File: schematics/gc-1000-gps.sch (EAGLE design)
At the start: 17 parts, among them T1 2N3904

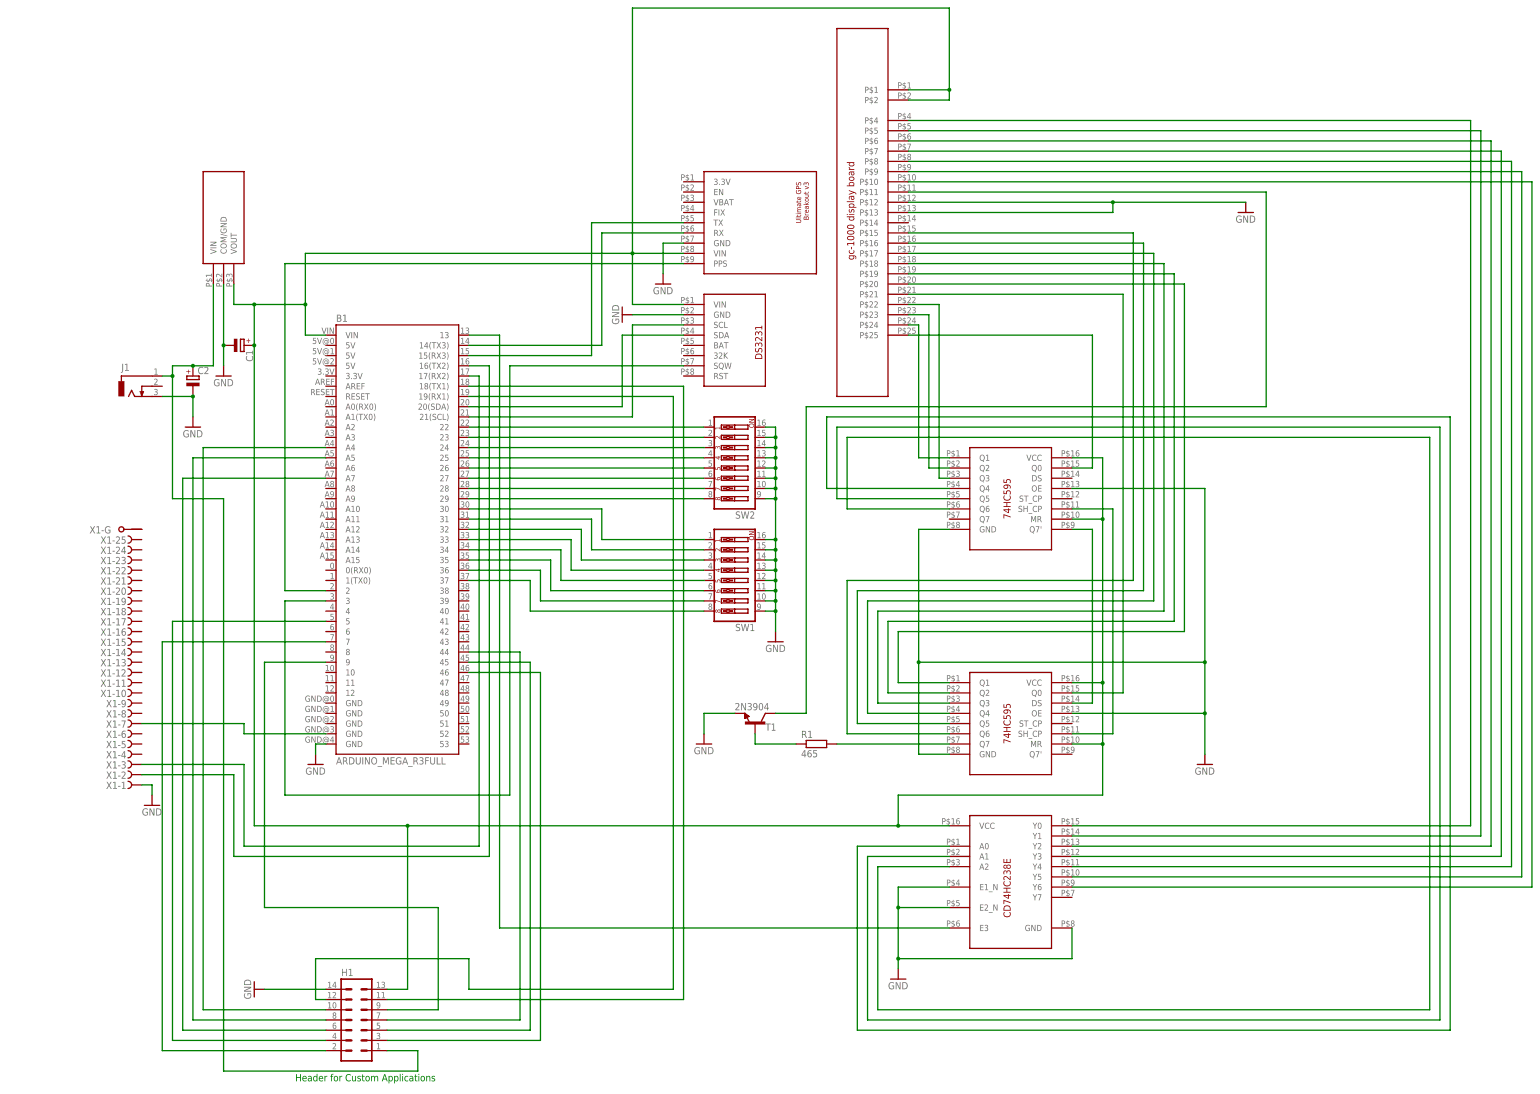
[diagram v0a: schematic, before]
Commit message: Import v0.2
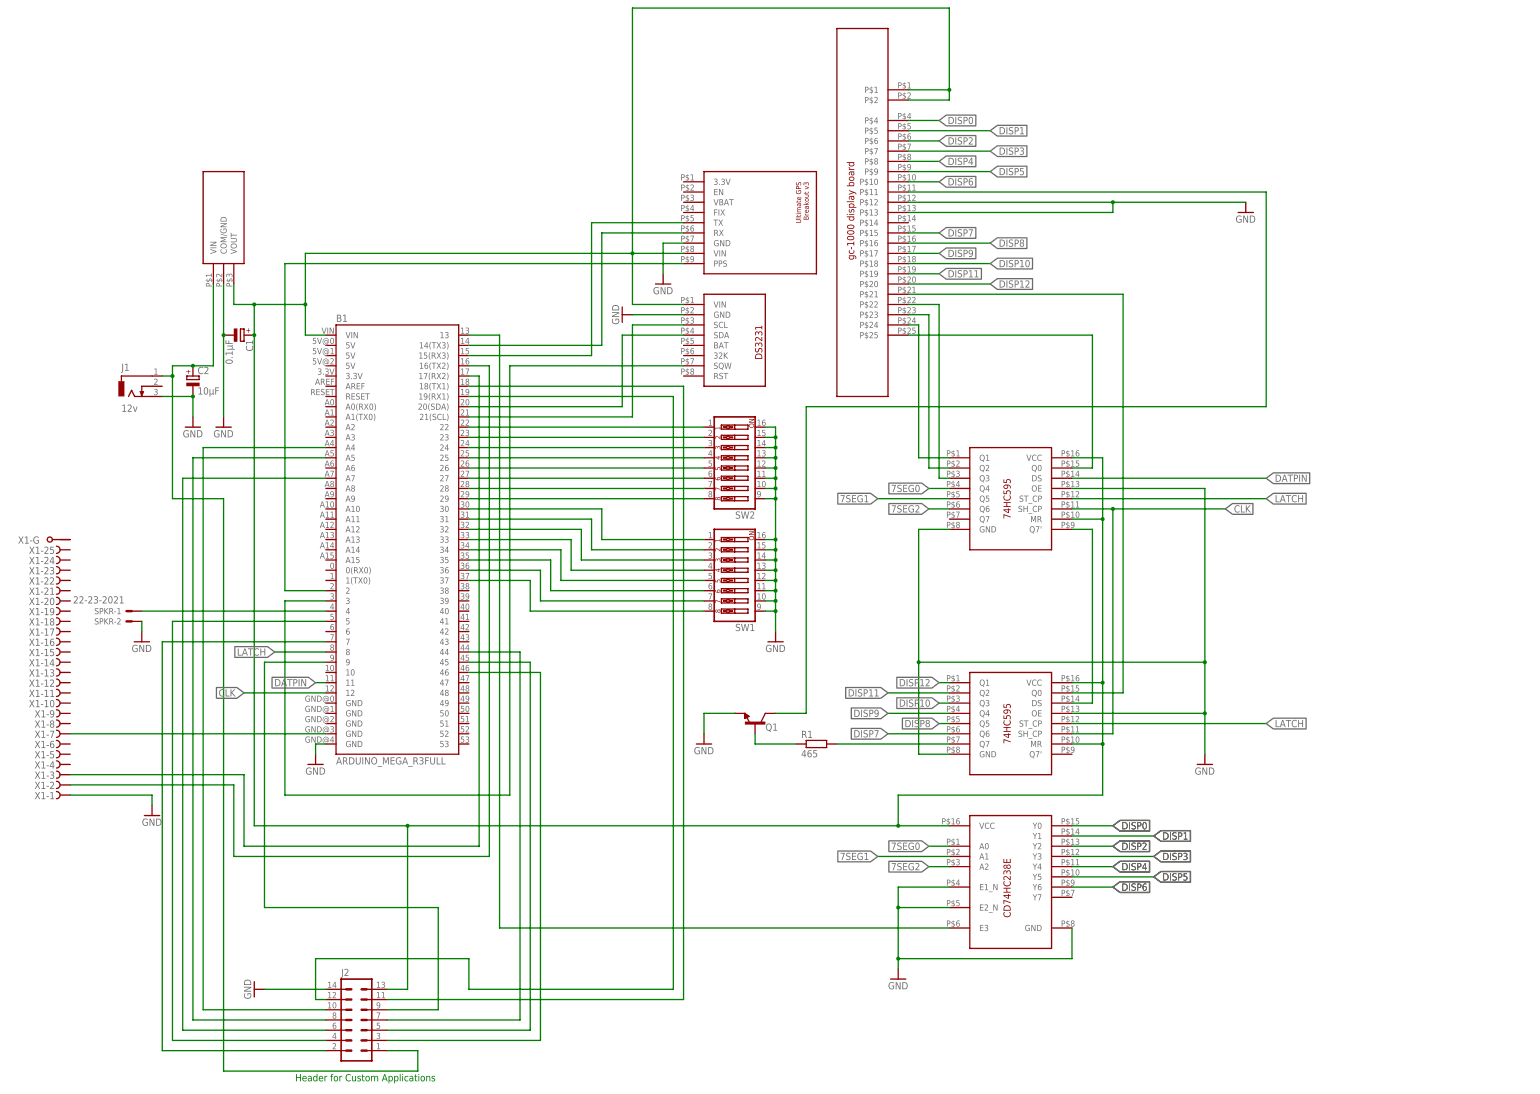
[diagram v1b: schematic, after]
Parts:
- added SPKR: 22-23-2021, con-molex:22-23-2021
- C1: value (none) -> 0.1µF
- C2: value (none) -> 10µF
- J1: value (none) -> 12v
- renumbered H1 to J2, T1 to Q1, U$3 to U1
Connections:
- net N$21 renamed DISP6
- net N$23 renamed DISP5
- net N$24 renamed DISP4
- net N$25 renamed DISP3
- net N$26 renamed DISP2
- net N$27 renamed DISP1
- net N$28 renamed DISP0
- net N$34 renamed DISP7
- net N$35 renamed DISP8
- net N$36 renamed DISP9
- net N$37 renamed DISP10
- net N$38 renamed DISP11
- net N$39 renamed DISP12
- net N$40 renamed 7SEG2
- net N$41 renamed 7SEG1
- net N$42 renamed 7SEG0
- removed net N$29: U$6.SH_CP, U$7.SH_CP
- new net CLK: B1.12, U$6.SH_CP, U$7.SH_CP
- new net DATPIN: B1.11, U$6.DS
- new net LATCH: B1.8, U$6.ST_CP, U$7.ST_CP
- new net N$21: B1.4, SPKR-1.S
- net GND: now also SPKR-2.S
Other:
- moved on the sheet: C1, X1-1, X1-10, X1-11, X1-12, X1-13, X1-14, X1-15, X1-16, X1-17, X1-18, X1-19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
